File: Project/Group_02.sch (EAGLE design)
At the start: 29 parts, among them J1 POWER_JACKPTH_LOCK, U1 +12v

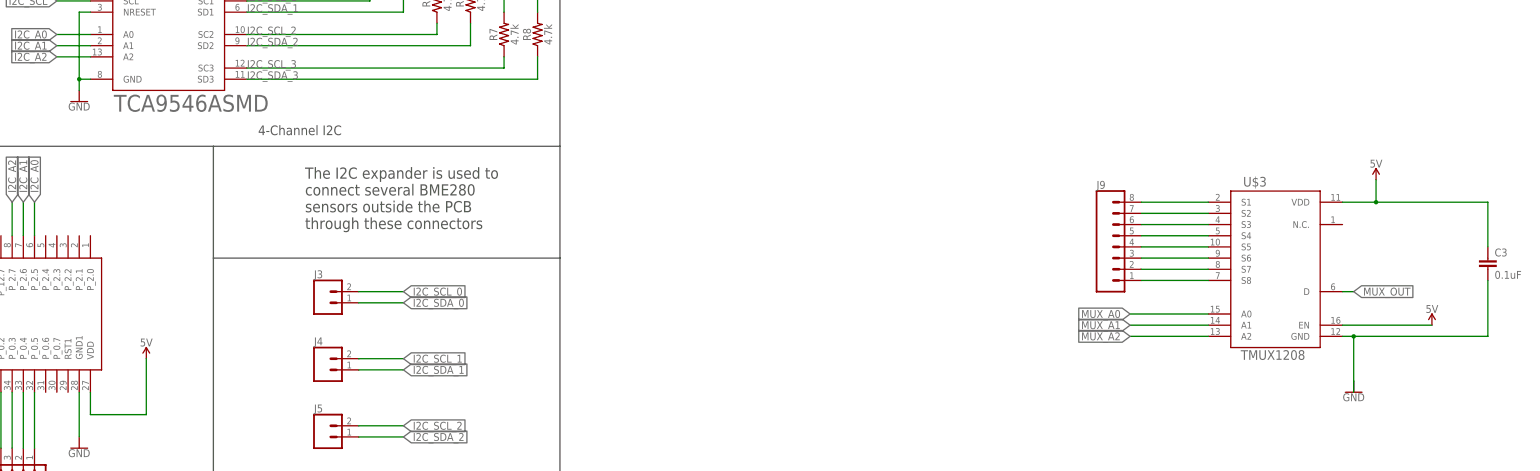
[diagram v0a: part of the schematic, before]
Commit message: Completamento board
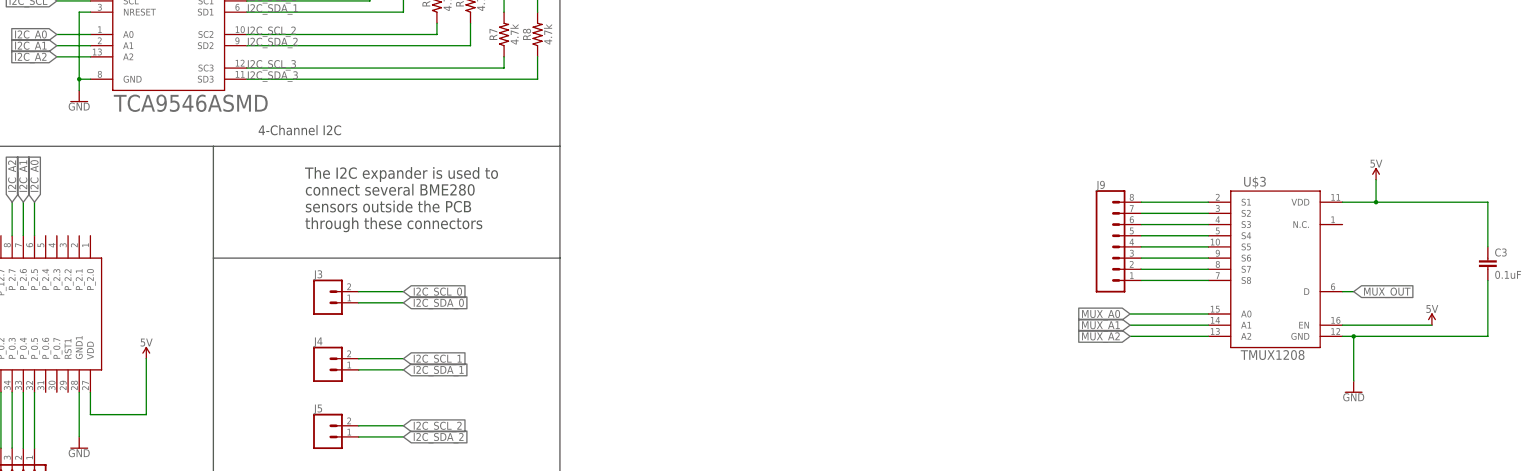
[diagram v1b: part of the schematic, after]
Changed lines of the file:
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@@
 <part name="SUPPLY8" library="SparkFun-PowerSymbols" deviceset="5V" device=""/>
 <part name="SUPPLY10" library="SparkFun-PowerSymbols" deviceset="5V" device=""/>
-<part name="GND1" library="SparkFun-PowerSymbols" deviceset="GND" device=""/>
 <part name="GND2" library="SparkFun-PowerSymbols" deviceset="GND" device=""/>
 <part name="GND3" library="SparkFun-PowerSymbols" deviceset="GND" device=""/>
@@
 <part name="SUPPLY12" library="SparkFun-PowerSymbols" deviceset="5V" device=""/>
 <part name="SUPPLY4" library="SparkFun-PowerSymbols" deviceset="5V" device=""/>
+<part name="GND1" library="SparkFun-PowerSymbols" deviceset="GND" device=""/>
 </parts>
 <sheets>
@@
 <attribute name="VALUE" x="472.44" y="81.534" size="1.778" layer="96" align="bottom-center"/>
 </instance>
-<instance part="GND1" gate="1" x="454.66" y="63.5" smashed="yes">
-<attribute name="VALUE" x="454.66" y="63.246" size="1.778" layer="96" align="top-center"/>
-</instance>
 <instance part="GND2" gate="1" x="165.1" y="50.8" smashed="yes">
 <attribute name="VALUE" x="165.1" y="50.546" size="1.778" layer="96" align="top-center"/>
@@
 <instance part="SUPPLY4" gate="G$1" x="162.56" y="175.26" smashed="yes">
 <attribute name="VALUE" x="162.56" y="178.054" size="1.778" layer="96" align="bottom-center"/>
+</instance>
+<instance part="GND1" gate="1" x="454.66" y="63.5" smashed="yes">
+<attribute name="VALUE" x="454.66" y="63.246" size="1.778" layer="96" align="top-center"/>
 </instance>
 </instances>
@@
 </segment>
 <segment>
-<pinref part="C3" gate="G$1" pin="2"/>
-<wire x1="485.14" y1="88.9" x2="485.14" y2="76.2" width="0.1524" layer="91"/>
-<wire x1="485.14" y1="76.2" x2="454.66" y2="76.2" width="0.1524" layer="91"/>
-<pinref part="U$3" gate="G$1" pin="GND"/>
-<pinref part="GND1" gate="1" pin="GND"/>
-<wire x1="454.66" y1="76.2" x2="452.12" y2="76.2" width="0.1524" layer="91"/>
-<wire x1="454.66" y1="66.04" x2="454.66" y2="63.5" width="0.1524" layer="91"/>
-<wire x1="454.66" y1="66.04" x2="454.66" y2="76.2" width="0.1524" layer="91"/>
-<junction x="454.66" y="76.2"/>
-</segment>
-<segment>
-<pinref part="U$2" gate="G$1" pin="GND"/>
 <pinref part="GND9" gate="1" pin="GND"/>
-<wire x1="167.64" y1="134.62" x2="165.1" y2="134.62" width="0.1524" layer="91"/>
-<wire x1="165.1" y1="134.62" x2="165.1" y2="132.08" width="0.1524" layer="91"/>
 <pinref part="U$2" gate="G$1" pin="NRESET"/>
+<wire x1="165.1" y1="132.08" x2="165.1" y2="134.62" width="0.1524" layer="91"/>
 <wire x1="165.1" y1="134.62" x2="165.1" y2="149.86" width="0.1524" layer="91"/>
 <wire x1="165.1" y1="149.86" x2="167.64" y2="149.86" width="0.1524" layer="91"/>
+<pinref part="U$2" gate="G$1" pin="GND"/>
+<wire x1="167.64" y1="134.62" x2="165.1" y2="134.62" width="0.1524" layer="91"/>
 <junction x="165.1" y="134.62"/>
 </segment>
+<segment>
+<pinref part="U$3" gate="G$1" pin="GND"/>
+<wire x1="452.12" y1="76.2" x2="454.66" y2="76.2" width="0.1524" layer="91"/>
+<wire x1="454.66" y1="76.2" x2="454.66" y2="66.04" width="0.1524" layer="91"/>
+<pinref part="GND1" gate="1" pin="GND"/>
+<wire x1="454.66" y1="76.2" x2="485.14" y2="76.2" width="0.1524" layer="91"/>
+<junction x="454.66" y="76.2"/>
+<pinref part="C3" gate="G$1" pin="2"/>
+<wire x1="485.14" y1="76.2" x2="485.14" y2="88.9" width="0.1524" layer="91"/>
+</segment>
 </net>
